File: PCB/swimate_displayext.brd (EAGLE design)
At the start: 69.5 x 34.3 mm, 55 parts, among them IC1 LPC11U24, T1 BSS84, T2 BSS84, U1 USD-SOCKETNEW, U5 DS3231MZ/V+T, U6 MAX1595EUA33+, U7 MAX1811ESA-T, U8 MAX16054AZT+T, U9 HC_05, Y1 12.000MHz

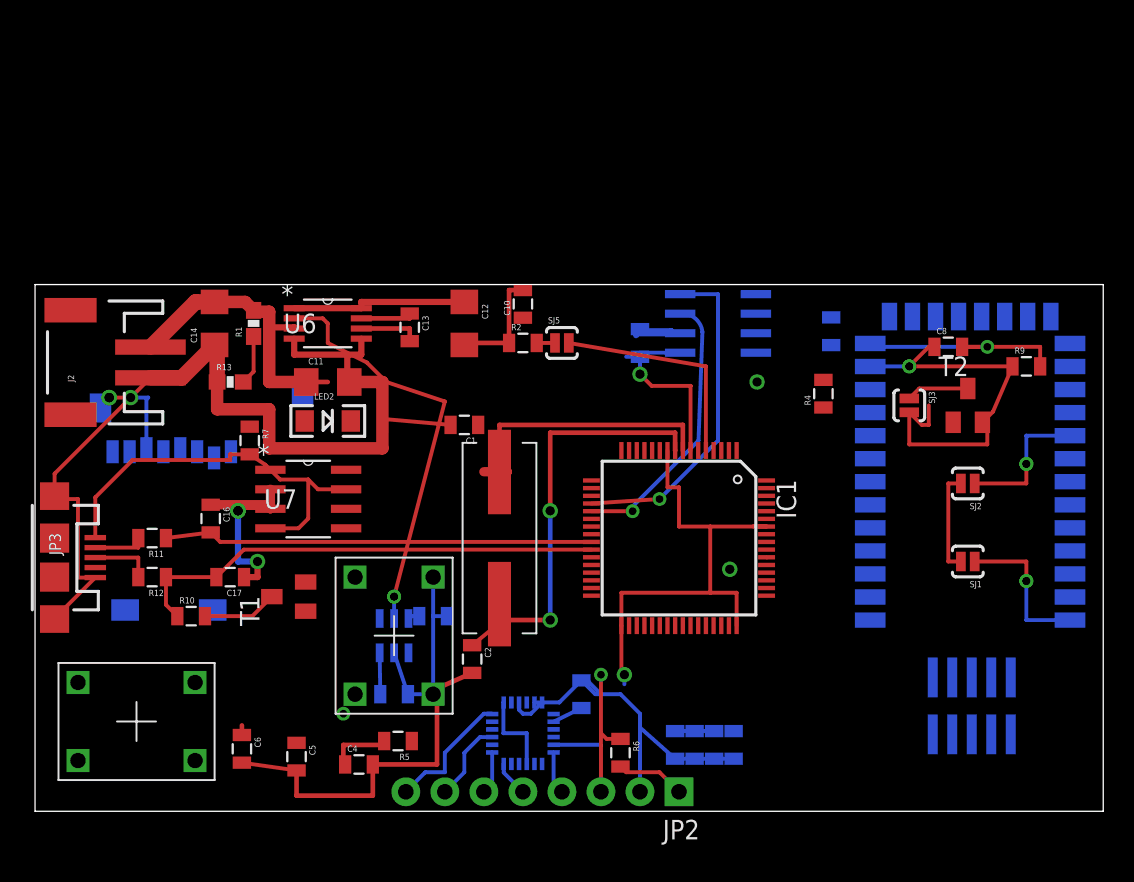
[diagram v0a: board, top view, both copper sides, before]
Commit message: Almost finished
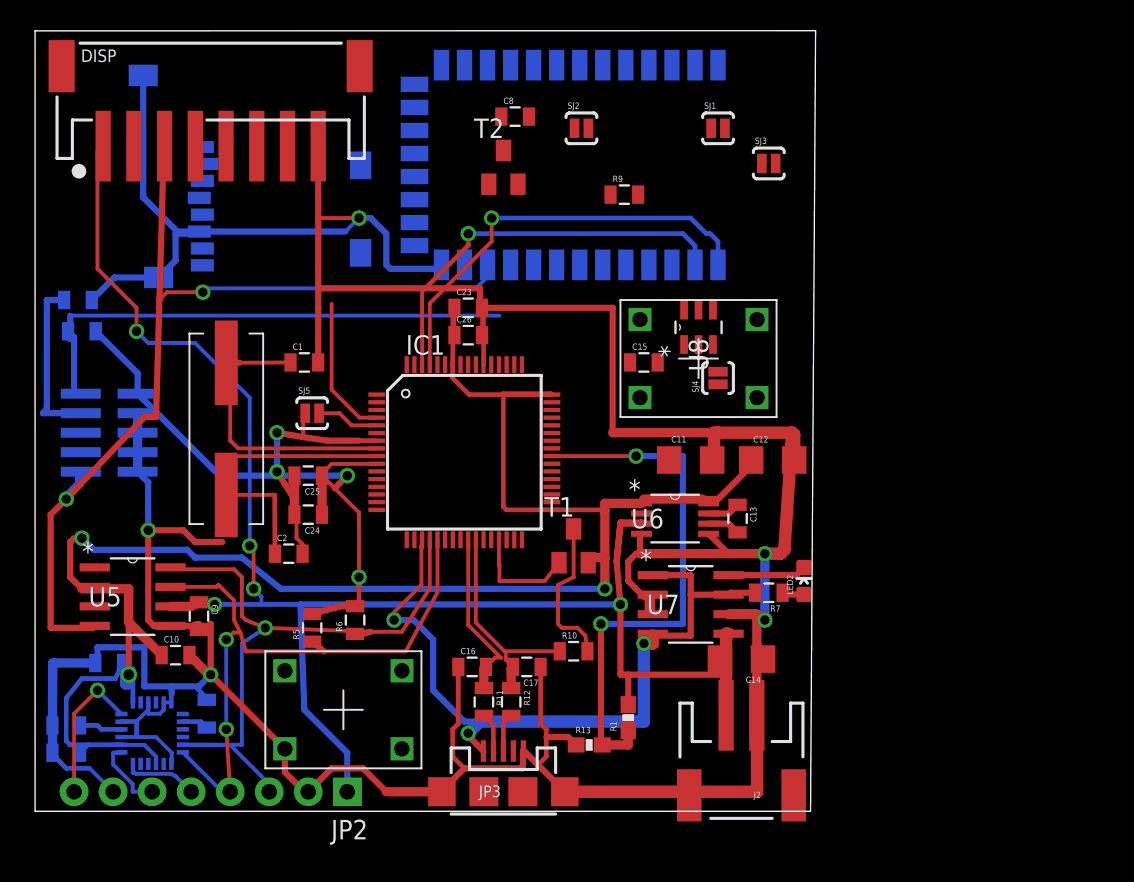
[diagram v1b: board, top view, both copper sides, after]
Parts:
- removed R2: 2k, SparkFun-Passives:0805
- removed R8: 24k, SparkFun-Passives:0805
- added DISP: (no value), microbuilder:JSTPH8
- added SJ4: SOLDERJUMPERNC2, SparkFun-Passives:SJ_2S-NOTRACE
- LED2: device SparkFun-LED:LED-1206 -> SparkFun-LED:LED-0603
- moved JTAG1 58.9 mm to (4.83, 24.6), turned to 270 degrees
- moved J2 49.9 mm to (46.0, 2.54), turned to 180 degrees
- moved R4 48.9 mm to (2.79, 33.3), flipped to the bottom, turned to 0 degrees
- moved R3 48.8 mm to (3.05, 31.2), turned to 180 degrees
- moved U5 42.0 mm to (6.35, 14.0), flipped to the top
- moved C14 40.7 mm to (46.0, 9.91), turned to 180 degrees
- moved R1 35.4 mm to (38.6, 6.10)
- moved R7 35.2 mm to (47.8, 14.2), turned to 180 degrees
- moved SJ2 34.2 mm to (35.6, 44.5), turned to 0 degrees
- moved T2 34.0 mm to (30.5, 41.9)
- moved C9 33.8 mm to (10.7, 12.7), flipped to the top
- moved R13 33.2 mm to (36.1, 4.32)
- moved JP3 32.9 mm to (30.5, 1.27), turned to 0 degrees
- moved LED2 32.7 mm to (50.0, 15.0)
- moved U9 32.6 mm to (40.6, 41.9), turned to 90 degrees
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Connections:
- net N$17 renamed USBD_P
- net N$18 renamed USBD_N
- net SWCLK renamed SCK0
- removed net MPU_AD0: JP2.7, U2.9
- removed net N$12: C12.1, U6.1, U6.8
- removed net N$21: R2.2, SJ5.1
- removed net N$4: C5.1, U2.13, U2.3
- removed net N$6: C23.1, C24.1, C25.1, C26.1, IC1.10, IC1.33, IC1.48, IC1.58
- removed net VBATTMON: R1.1, R13.2
- new net DISP_CS: DISP.5
- new net DISP_DC: DISP.7
- new net VBATMON: IC1.40, R1.1, R13.2
- net 3.3V: now also C12.1, C23.1, C24.1, C25.1, C26.1, C5.1, DISP.2, IC1.10, IC1.33, IC1.48, IC1.58, U2.13, U2.3, U6.1, U6.8; no longer JP2.1
- net GND: now also DISP.8, JP2.7, SJ4.1, SJ5.1, U2.1, U2.11, U2.9; no longer R2.1, R8.2, SW_MODE.P$1, SW_PWR.P$1
- net N$1: no longer SW_PWR.P$3
- net RST: now also DISP.3
- net SPI0_MOSI: now also DISP.6
- net SPI0_SCK: now also DISP.4
- net SW_MODE: no longer SW_MODE.P$3
- net SYS_SHUTDOWN: now also SJ4.2; no longer R8.1
- net VBAT: now also C15.1, DISP.1, JP2.1, U8.6
- net VUSB: no longer C15.1, U8.6
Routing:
- net 3.3V: track 12.9 -> 168.4 mm, vias 0 -> 5
- net GND: track 185.2 -> 316.7 mm
- net VBAT: track 26.7 -> 109.6 mm, vias 0 -> 5
- net RST: track 0.00 -> 73.9 mm, vias 0 -> 2
- net N$6: track 37.4 -> 0.00 mm, vias 1 -> 0
- net VBATMON: track 0.00 -> 35.3 mm, vias 0 -> 2
- net SWDIO: track 0.00 -> 34.7 mm
- net MCU_RX: track 0.00 -> 28.1 mm, vias 0 -> 1
- net N$15: track 27.2 -> 0.00 mm, vias 1 -> 0
- net 3V3_ENABLE: track 26.8 -> 0.00 mm, vias 1 -> 0
- net MCU_TX: track 0.00 -> 26.1 mm, vias 0 -> 1
- net VUSB: track 27.2 -> 49.9 mm, vias 0 -> 3
- net I2C_SDA: track 20.8 -> 42.4 mm, vias 2 -> 3
- net USBD_P: track 31.3 -> 14.3 mm
- net USBD_N: track 28.0 -> 11.2 mm
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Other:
- board size 69.5 x 34.3 mm -> 50.8 x 50.8 mm
